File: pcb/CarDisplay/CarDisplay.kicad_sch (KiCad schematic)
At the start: 13 parts, among them J1 Switch, J2 Display1, J3 Display2, J4 ECU_RS232, J5 SpeedSensor, U1 MAX3232

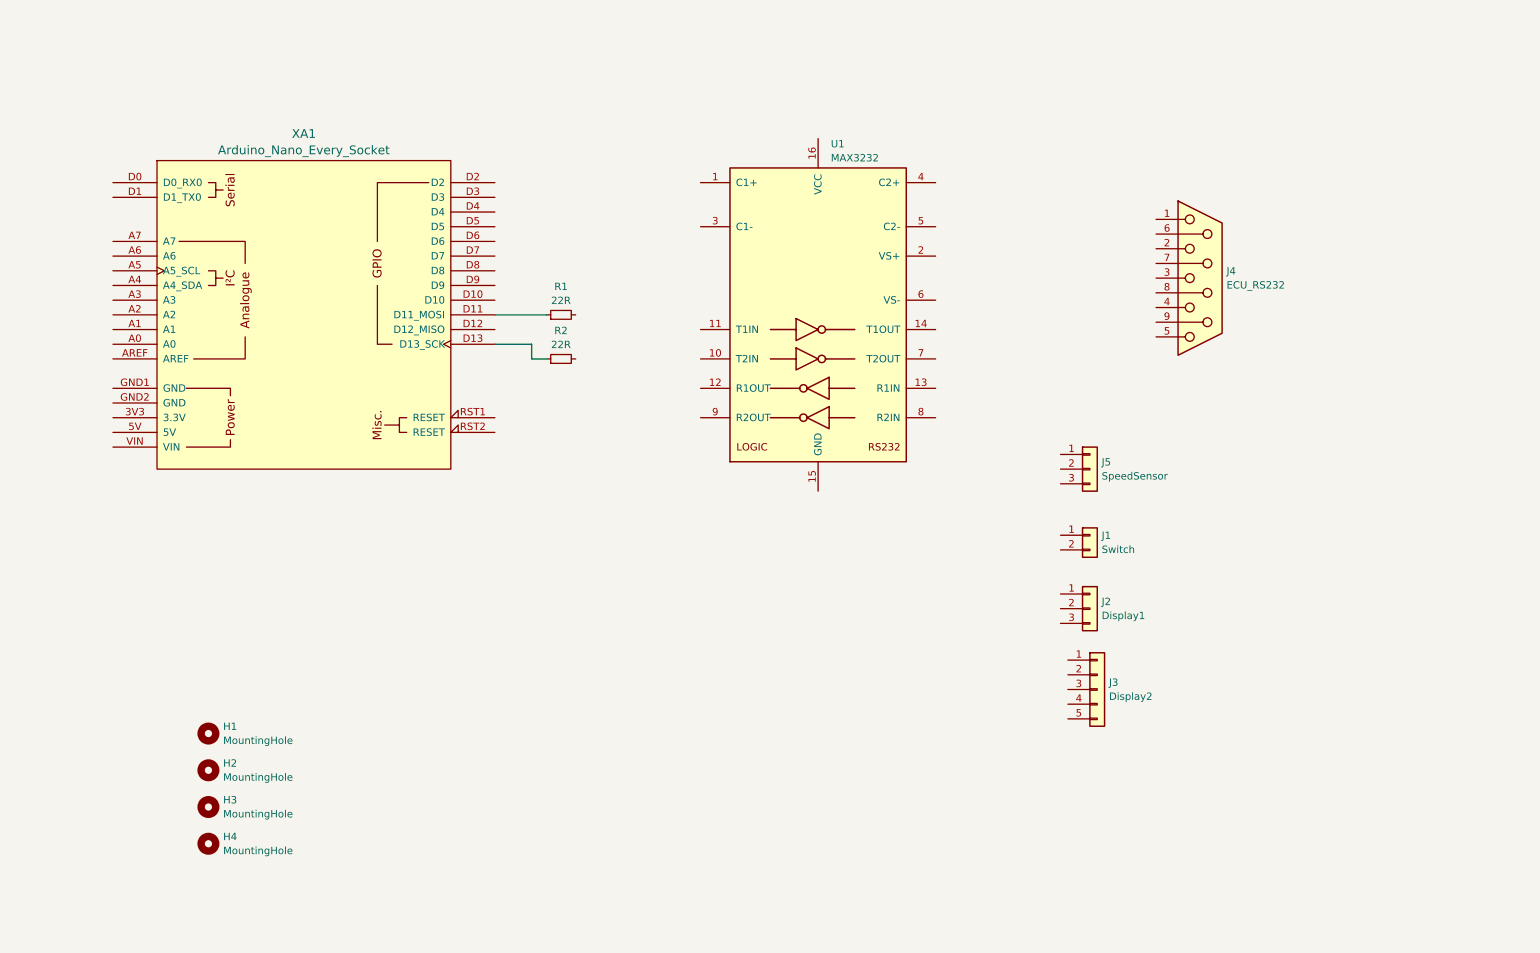
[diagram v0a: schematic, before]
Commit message: pcb dev
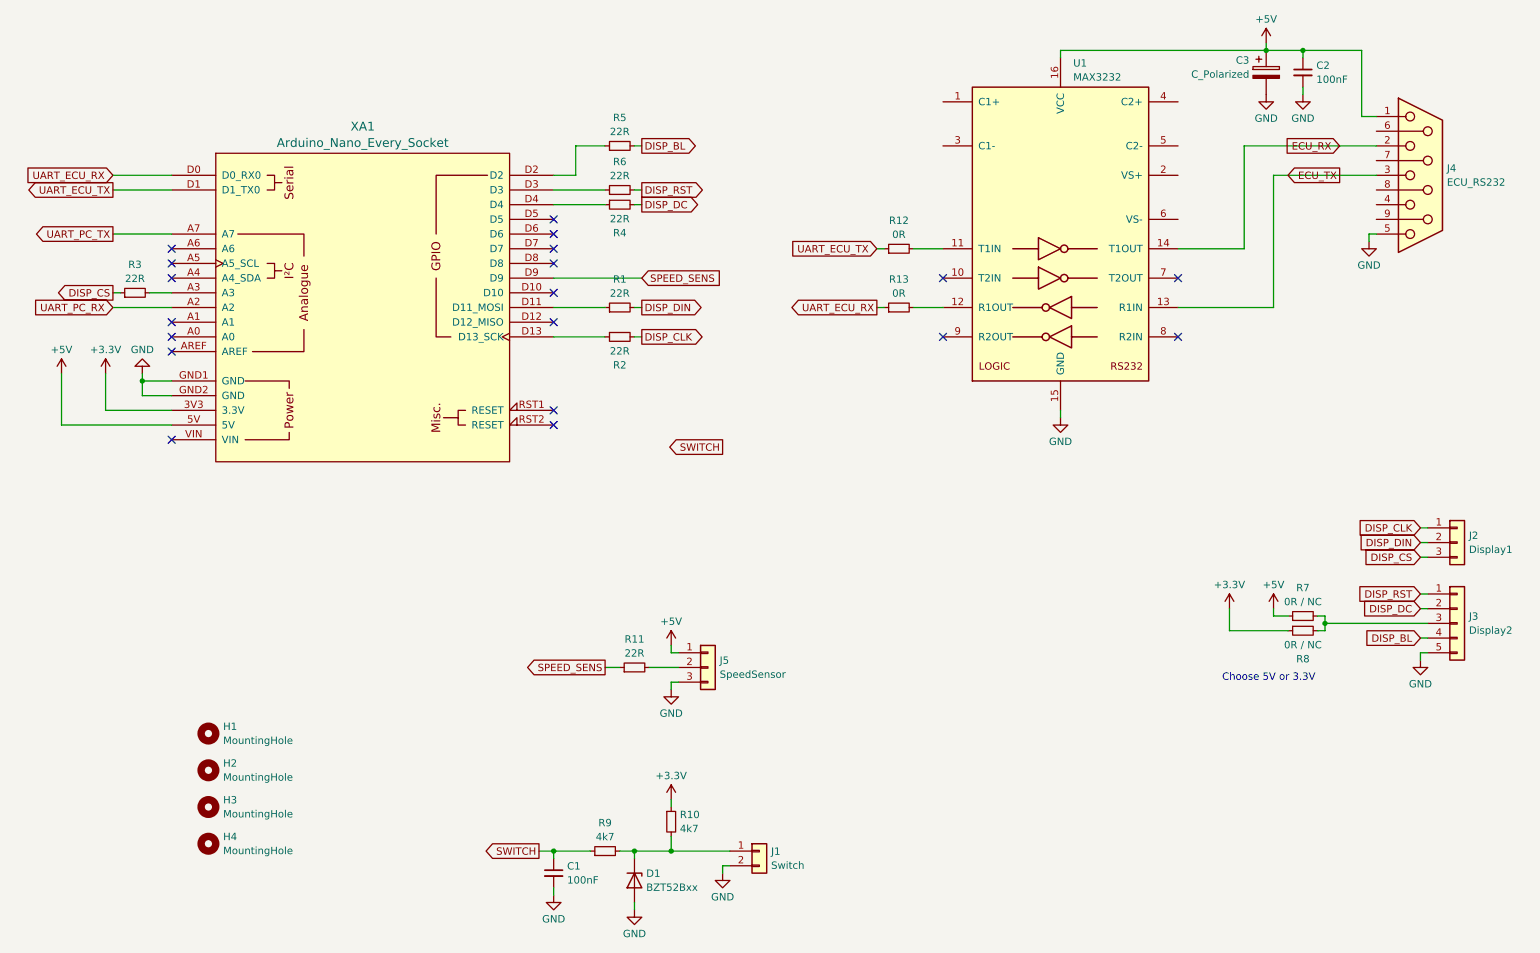
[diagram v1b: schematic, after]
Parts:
- added C1, C2: 100nF, Capacitor_SMD:C_1206_3216Metric_Pad1.33x1.80mm_HandSolder, symbol Device:C_Small
- added C3: C_Polarized, symbol Device:C_Polarized
- added D1: BZT52Bxx, Diode_SMD:D_SOD-123F, symbol Diode:BZT52Bxx
- added R10, R9: 4k7, Resistor_SMD:R_0805_2012Metric_Pad1.20x1.40mm_HandSolder, symbol Device:R_Small
- added R11, R3, R4, R5, R6: 22R, Resistor_SMD:R_0805_2012Metric_Pad1.20x1.40mm_HandSolder, symbol Device:R_Small
- added R12, R13: 0R, Resistor_SMD:R_0805_2012Metric_Pad1.20x1.40mm_HandSolder, symbol Device:R_Small
- added R7, R8: 0R / NC, Resistor_SMD:R_0805_2012Metric_Pad1.20x1.40mm_HandSolder, symbol Device:R_Small
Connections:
- net at U1.11 (T1IN): now also R12.2
- net at U1.12 (R1OUT): now also R13.2
- net ECU_TX: now reaches U1.13 (R1IN)
- net ECU_TX: now also J4.3
- net ECU_RX: now reaches U1.14 (T1OUT)
- net ECU_RX: now also J4.2
- net GND: now reaches U1.15 (GND)
- net GND: now also J1.2 (Pin_2), J3.5 (Pin_5), J4.5, J5.3 (Pin_3), XA1.GND1 (GND), XA1.GND2 (GND), C1.2, C2.2, C3.2, D1.2 (A)
- net +5V: now reaches U1.16 (VCC)
- net +5V: now also J4.1, J5.1 (Pin_1), XA1.5V, C2.1, C3.1, R7.1
- net DISP_CLK: now reaches J2.1 (Pin_1)
- net DISP_CLK: now also R2.2
- net DISP_DIN: now reaches J2.2 (Pin_2)
- net DISP_DIN: now also R1.2
- net DISP_CS: now reaches J2.3 (Pin_3)
- net DISP_CS: now also R3.1
- net at J1.1 (Pin_1): now also D1.1 (K), R10.2, R9.2
- net at J5.2 (Pin_2): now also R11.2
- net DISP_RST: now reaches J3.1 (Pin_1)
- net DISP_RST: now also R6.2
- net DISP_DC: now reaches J3.2 (Pin_2)
- net DISP_DC: now also R4.2
- net at J3.3 (Pin_3): now also R7.2, R8.2
- net DISP_BL: now reaches J3.4 (Pin_4)
- net DISP_BL: now also R5.2
- net +3.3V: now reaches XA1.3V3 (3.3V)
- net +3.3V: now also R10.1, R8.1
- net UART_PC_RX: now reaches XA1.A2
- net at XA1.A3: now also R3.2
- net UART_PC_TX: now reaches XA1.A7
- net UART_ECU_RX: now reaches XA1.D0 (D0_RX0)
- net UART_ECU_RX: now also R13.1
- net UART_ECU_TX: now reaches XA1.D1 (D1_TX0)
- net UART_ECU_TX: now also R12.1
- net at XA1.D2: now also R5.1
- net at XA1.D3: now also R6.1
- net at XA1.D4: now also R4.1
- net SPEED_SENS: now reaches XA1.D9
- net SPEED_SENS: now also R11.1
- new net SWITCH: C1.1, R9.1
- no-connect marks 0 -> 19
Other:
- note added: "Choose 5V or 3.3V"
- moved on the sheet: J1, J2, J3, J4, J5, R1, R2, U1, XA1
